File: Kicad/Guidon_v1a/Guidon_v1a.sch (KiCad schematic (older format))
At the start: 42 parts, among them IC1 L7805CDT, IC2 DSPIC30F4012, IC3 AMS1117-3.3, IC4 MCP2562, K1 ICSP, K2 ALIM, K3 BUS CAN, K4 GUIDON G, K5 FREIN, K6 AFF OLED, K7 GUIDON D, K8 RESERVE, K9 BP OLED, X1 8M

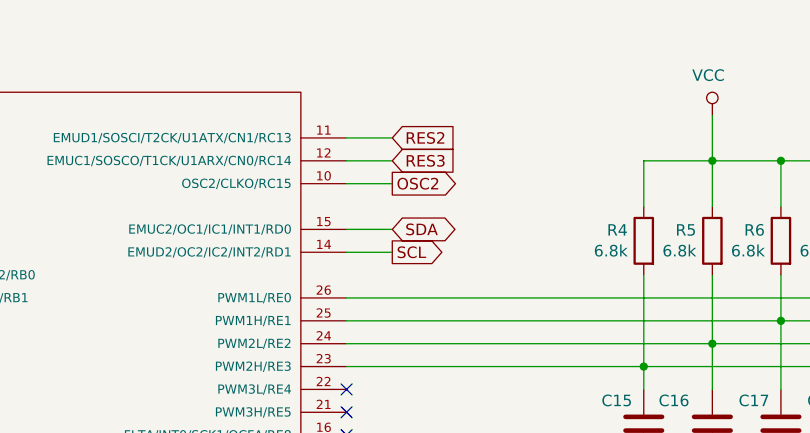
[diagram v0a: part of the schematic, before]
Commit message: Update
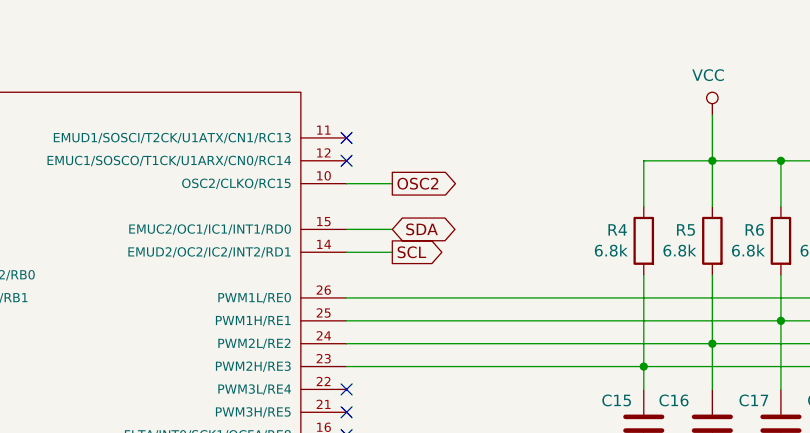
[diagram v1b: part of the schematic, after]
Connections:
- net RES2: no longer names the net of IC2.11 (EMUD1/SOSCI/T2CK/U1ATX/CN1/RC13)
- net RES3: no longer names the net of IC2.12 (EMUC1/SOSCO/T1CK/U1ARX/CN0/RC14)
- no-connect marks 6 -> 8
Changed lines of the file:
@@
 	3350 7400 3350 7200
-Wire Wire Line
-	4700 1600 4900 1600
-Wire Wire Line
-	4700 1500 4900 1500
-Text GLabel 4900 1500 2    50   Input ~ 0
-RES2
-Text GLabel 4900 1600 2    50   Input ~ 0
-RES3
 Wire Wire Line
 	900  2800 1100 2800
@@
 Wire Wire Line
 	2800 5200 2800 5000
+NoConn ~ 4700 1500
+NoConn ~ 4700 1600
 $EndSCHEMATC
